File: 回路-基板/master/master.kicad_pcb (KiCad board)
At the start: 2 copper layers, 23 parts, among them J1 Ext. PWR, J2 Conn_01x07_Pin, SW1 SW_SPDT, SW2 SW_SPDT, SW3 RESET, U1 TWE-L-DP-W, U2 LM1117MP-3.3, U3 DEV-16771

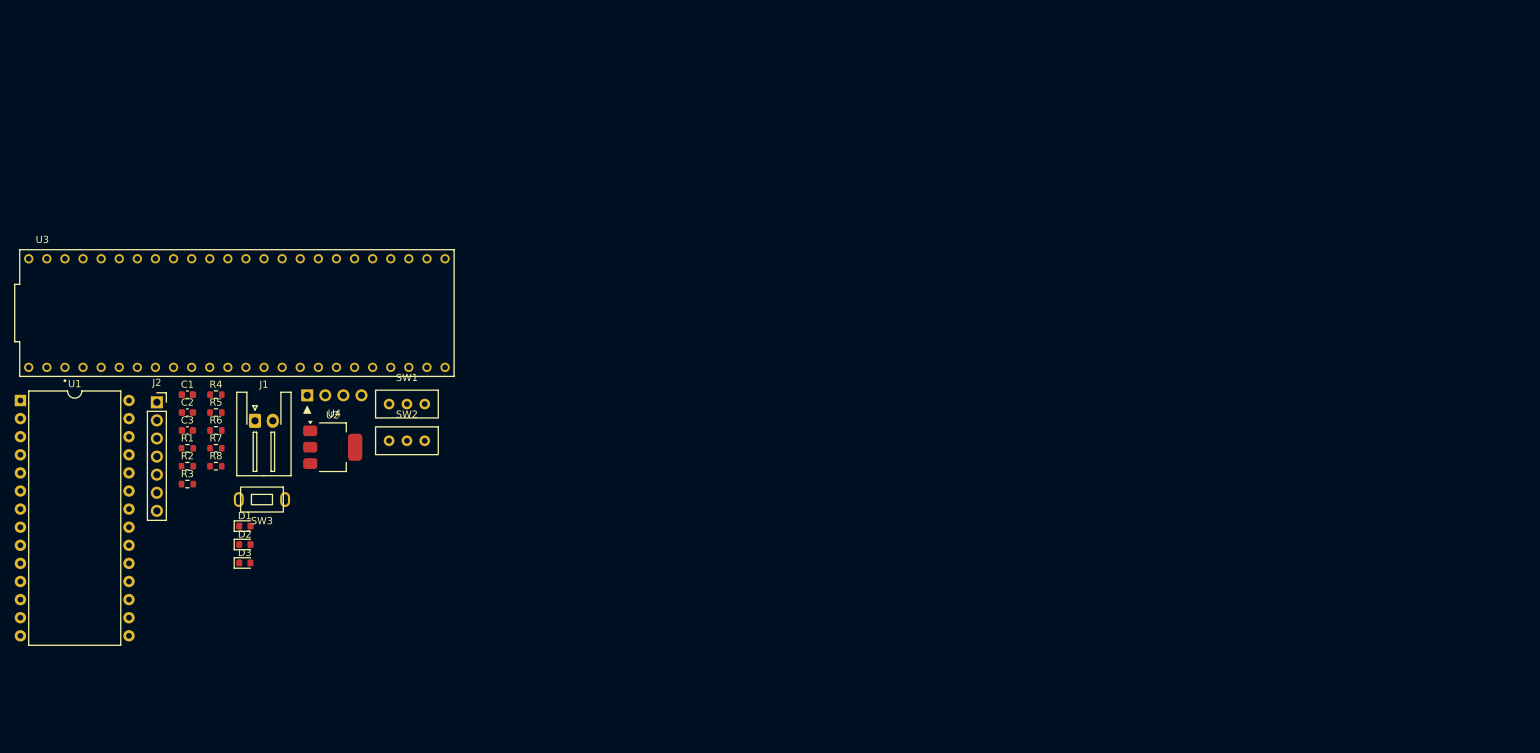
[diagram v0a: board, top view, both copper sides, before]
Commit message: PCB_1
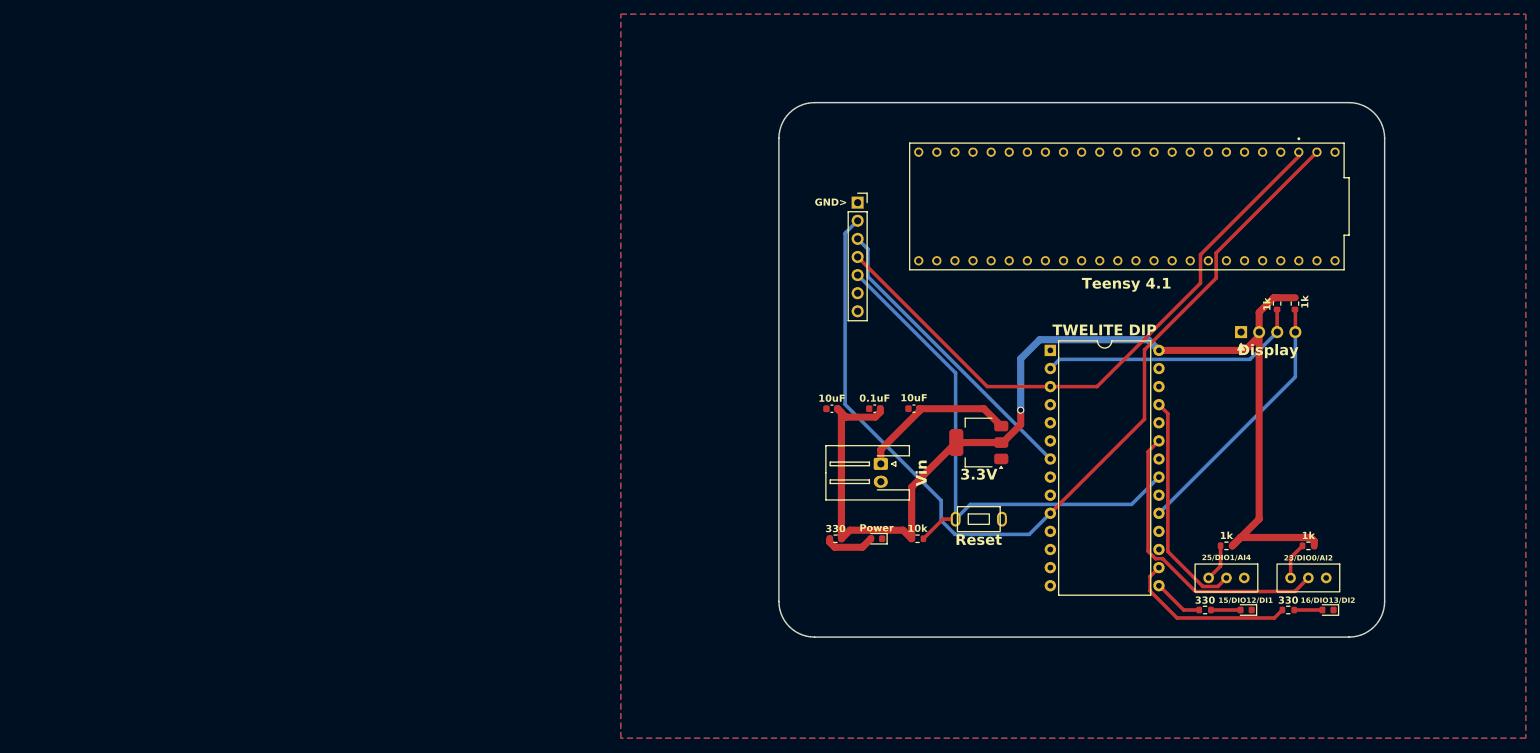
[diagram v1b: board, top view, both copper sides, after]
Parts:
- removed C1, C3: 10uF, Capacitor_SMD:C_0603_1608Metric
- removed C2: 0.1uF, Capacitor_SMD:C_0603_1608Metric
- removed D1: PWR, LED_SMD:LED_0603_1608Metric
- removed D2: LED1, LED_SMD:LED_0603_1608Metric
- removed D3: LED2, LED_SMD:LED_0603_1608Metric
- removed J1: Ext. PWR, Connector_JST:JST_XH_S2B-XH-A-1_1x02_P2.50mm_Horizontal
- removed J2: Conn_01x07_Pin, Connector_PinSocket_2.54mm:PinSocket_1x07_P2.54mm_Vertical
- removed R1, R2, R3: 330, Resistor_SMD:R_0603_1608Metric
- removed R5: 1K, Resistor_SMD:R_0603_1608Metric
- removed R6: 10K, Resistor_SMD:R_0603_1608Metric
- removed R7, R8: R_Small, Resistor_SMD:R_0603_1608Metric
- removed SW1, SW2: SW_SPDT, @2024-cansat:SS12D01G4
- removed SW3: RESET, @2024-cansat:TVBP06-B043C
- removed U1: TWE-L-DP-W, Package_DIP:DIP-28_W15.24mm
- removed U2: LM1117MP-3.3, Package_TO_SOT_SMD:SOT-223-3_TabPin2
- removed U3: DEV-16771, @2024-cansat:MODULE_DEV-16771
- removed U4: ~, @2024-cansat:Display
- added 0.1uF: 0.1uF, Capacitor_SMD:C_0603_1608Metric, F.Cu at (162.7, 80.8)
- added 10k: 10K, Resistor_SMD:R_0603_1608Metric, F.Cu at (168.7, 99.0)
- added 10uF: 10uF, Capacitor_SMD:C_0603_1608Metric, F.Cu at (168.2, 80.8)
- added 10uF: 10uF, Capacitor_SMD:C_0603_1608Metric, F.Cu at (156.6, 80.8)
- added 15/DIO12/DI1: LED1, LED_SMD:LED_0603_1608Metric, F.Cu at (214.8, 109.0)
- added 16/DIO13/DI2: LED2, LED_SMD:LED_0603_1608Metric, F.Cu at (226.2, 109.0)
- added 1k: 1K, Resistor_SMD:R_0603_1608Metric, F.Cu at (221.6, 66.0)
- added 1k: R_Small, Resistor_SMD:R_0603_1608Metric, F.Cu at (212.0, 100.0)
- added 1k: R_Small, Resistor_SMD:R_0603_1608Metric, F.Cu at (223.5, 100.0)
- added 23/DIO0/AI2: SW_SPDT, 2024-cansat:SS12D01G4, F.Cu at (223.5, 104.5)
- added 25/DIO1/AI4: SW_SPDT, 2024-cansat:SS12D01G4, F.Cu at (212.0, 104.5)
- added 3.3V: LM1117MP-3.3, Package_TO_SOT_SMD:SOT-223-3_TabPin2, F.Cu at (177.2, 85.5)
- added 330: 330, Resistor_SMD:R_0603_1608Metric, F.Cu at (220.7, 109.0)
- added 330: 330, Resistor_SMD:R_0603_1608Metric, F.Cu at (157.2, 99.0)
- added 330: 330, Resistor_SMD:R_0603_1608Metric, F.Cu at (209.0, 109.0)
- added Display: ~, 2024-cansat:Display, F.Cu at (217.9, 70.0)
- added GND>: Conn_01x07_Pin, Connector_PinSocket_2.54mm:PinSocket_1x07_P2.54mm_Vertical, F.Cu at (160.2, 51.8)
- added Power: PWR, LED_SMD:LED_0603_1608Metric, F.Cu at (162.9, 99.0)
- added Reset: RESET, 2024-cansat:TVBP06-B043C, F.Cu at (177.2, 96.2)
- added TWELITE DIP: TWE-L-DP-W, Package_DIP:DIP-28_W15.24mm, F.Cu at (187.3, 72.6)
- added Teensy 4.1: DEV-16771, 2024-cansat:MODULE_DEV-16771, F.Cu at (198.0, 52.4)
- added Vin: Ext. PWR, Connector_JST:JST_XH_S2B-XH-A-1_1x02_P2.50mm_Horizontal, F.Cu at (163.5, 88.5)
- moved R4 149.5 mm to (219.1, 66.0), turned to 90 degrees
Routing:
- net +3.3V: track 0.00 -> 161.6 mm, vias 0 -> 1
- net 10: track 0.00 -> 131.9 mm
- net 3: track 0.00 -> 85.8 mm
- net 21: track 0.00 -> 76.6 mm
- net 7: track 0.00 -> 42.1 mm
- net 23: track 0.00 -> 41.7 mm
- net 2: track 0.00 -> 37.1 mm
- net 19: track 0.00 -> 36.6 mm
- net 25: track 0.00 -> 31.9 mm
- net 16: track 0.00 -> 24.4 mm
- net Net-(J1-Pin_1): track 0.00 -> 22.5 mm
- net Net-(D1-A): track 0.00 -> 7.06 mm
- net 15: track 0.00 -> 7.06 mm
- net Net-(SW2-A): track 0.00 -> 5.19 mm
- net Net-(SW1-A): track 0.00 -> 5.19 mm
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- added copper zone on B.Cu, net GND
- added copper zone on F.Cu, net GND
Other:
- board outline added: 85 x 75 mm
- board text added: "1k"

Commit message: PCB進めた
発注用ファイルも作成した
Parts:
- removed 0.1uF: 0.1uF, Capacitor_SMD:C_0603_1608Metric
- removed 10k: 10K, Resistor_SMD:R_0603_1608Metric
- removed 10uF (x2): 10uF, Capacitor_SMD:C_0603_1608Metric
- removed 1k: 1K, Resistor_SMD:R_0603_1608Metric
- removed 1k (x2): R_Small, Resistor_SMD:R_0603_1608Metric
- removed 330 (x3): 330, Resistor_SMD:R_0603_1608Metric
- added C1: 10uF, Capacitor_SMD:C_0603_1608Metric, F.Cu at (-40.3, -20.4)
- added C2: 0.1uF, Capacitor_SMD:C_0603_1608Metric, F.Cu at (-12.6, -28.7)
- added C3: 10uF, Capacitor_SMD:C_0603_1608Metric, F.Cu at (-40.3, -9.43)
- added R1: 330, Resistor_THT:R_Axial_DIN0207_L6.3mm_D2.5mm_P7.62mm_Horizontal, F.Cu at (-53.7, -4.41)
- added R2: 330, Resistor_THT:R_Axial_DIN0207_L6.3mm_D2.5mm_P7.62mm_Horizontal, F.Cu at (-10.3, 6.00)
- added R3: 330, Resistor_THT:R_Axial_DIN0207_L6.3mm_D2.5mm_P7.62mm_Horizontal, F.Cu at (2.69, 6.00)
- added R5: 1K, Resistor_THT:R_Axial_DIN0207_L6.3mm_D2.5mm_P7.62mm_Horizontal, F.Cu at (3.81, -37.0)
- added R6: 10K, Resistor_THT:R_Axial_DIN0207_L6.3mm_D2.5mm_P7.62mm_Horizontal, F.Cu at (-50.2, -4.41)
- added R7: R_Small, Resistor_THT:R_Axial_DIN0207_L6.3mm_D2.5mm_P7.62mm_Horizontal, F.Cu at (-10.3, -4.00)
- added R8: R_Small, Resistor_THT:R_Axial_DIN0207_L6.3mm_D2.5mm_P7.62mm_Horizontal, F.Cu at (2.69, -4.00)
- R4: footprint Resistor_SMD:R_0603_1608Metric -> Resistor_THT:R_Axial_DIN0207_L6.3mm_D2.5mm_P7.62mm_Horizontal
- moved 23/DIO0/AI2 252.6 mm to (-6.50, 0.00)
- moved 15/DIO12/DI1 242.6 mm to (-6.50, 9.50), turned to 0 degrees
- moved Teensy 4.1 242.5 mm to (-22.6, -48.1)
- moved 16/DIO13/DI2 241.2 mm to (6.50, 9.50), turned to 0 degrees
- moved GND> 239.9 mm to (-57.6, -48.7)
- moved Reset 239.9 mm to (-40.6, -4.25)
- moved Vin 239.9 mm to (-54.4, -12.0)
- moved TWELITE DIP 239.9 mm to (-30.6, -27.9)
- moved 3.3V 239.8 mm to (-40.5, -14.9)
- moved Display 238.7 mm to (0.00, -27.5)
- moved R4 237.4 mm to (3.81, -34.0), turned to 180 degrees
- moved Power 235.4 mm to (-53.7, 6.65), turned to 90 degrees
- moved 25/DIO1/AI4 230.5 mm to (6.50, 0.00)
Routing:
- net 23: track 41.7 -> 18.9 mm
- net 16: track 24.4 -> 19.5 mm
- net 19: track 36.6 -> 41.0 mm
- net Net-(D1-A): track 7.06 -> 2.65 mm
- net 21: track 76.6 -> 81.0 mm
- net 2: track 37.1 -> 41.3 mm
- net 15: track 7.06 -> 5.40 mm
- net 25: track 31.9 -> 33.2 mm
- net Net-(J1-Pin_1): track 22.5 -> 21.2 mm
- net 3: track 85.8 -> 84.6 mm
- net 10: track 131.9 -> 130.9 mm
- net Net-(D3-A): track 3.96 -> 4.75 mm
- net Net-(SW2-A): track 5.19 -> 4.54 mm
- net Net-(SW1-A): track 5.19 -> 4.54 mm
- net Net-(D2-A): track 4.14 -> 4.75 mm
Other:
- board text added: "0.1uF"
- board text added: "10k"
- board text added: "10uF"
- board text added: "330"
- board text added: "USB"
